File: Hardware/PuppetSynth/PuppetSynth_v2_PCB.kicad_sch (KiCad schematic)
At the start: 59 parts, among them J10 PINHD_1x6_Female, J11 JST_03, J12 JST_03, J13 JST_05, J14 JST_05, J15 JST_05, J16 JST_03, J17 JST_03, J18 JST_03, J19 PINHD_1x6_Female, J20 JST_03, J21 JST_03, J22 JST_03, J24 JST_03, J25 JST_03, J26 JST_03, J3 JST_03, J4 JST_03, J5 JST_05, J6 JST_05, J7 JST_05, J8 PINHD_1x6_Female, J9 PINHD_1x6_Female

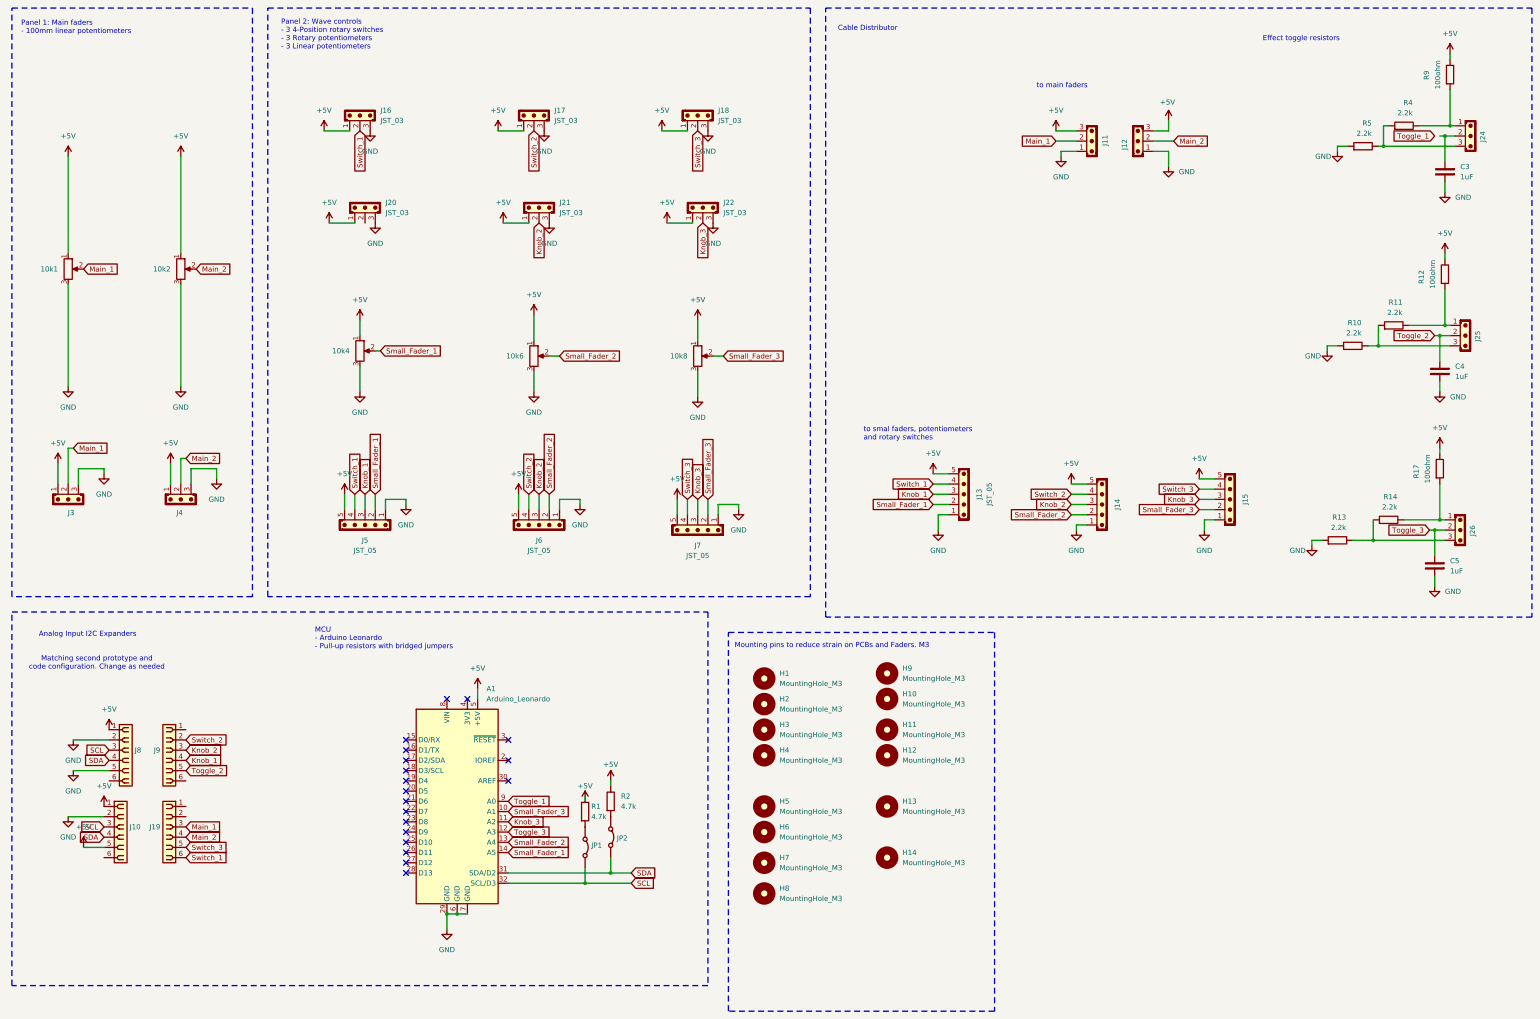
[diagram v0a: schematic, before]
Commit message: updated pcb
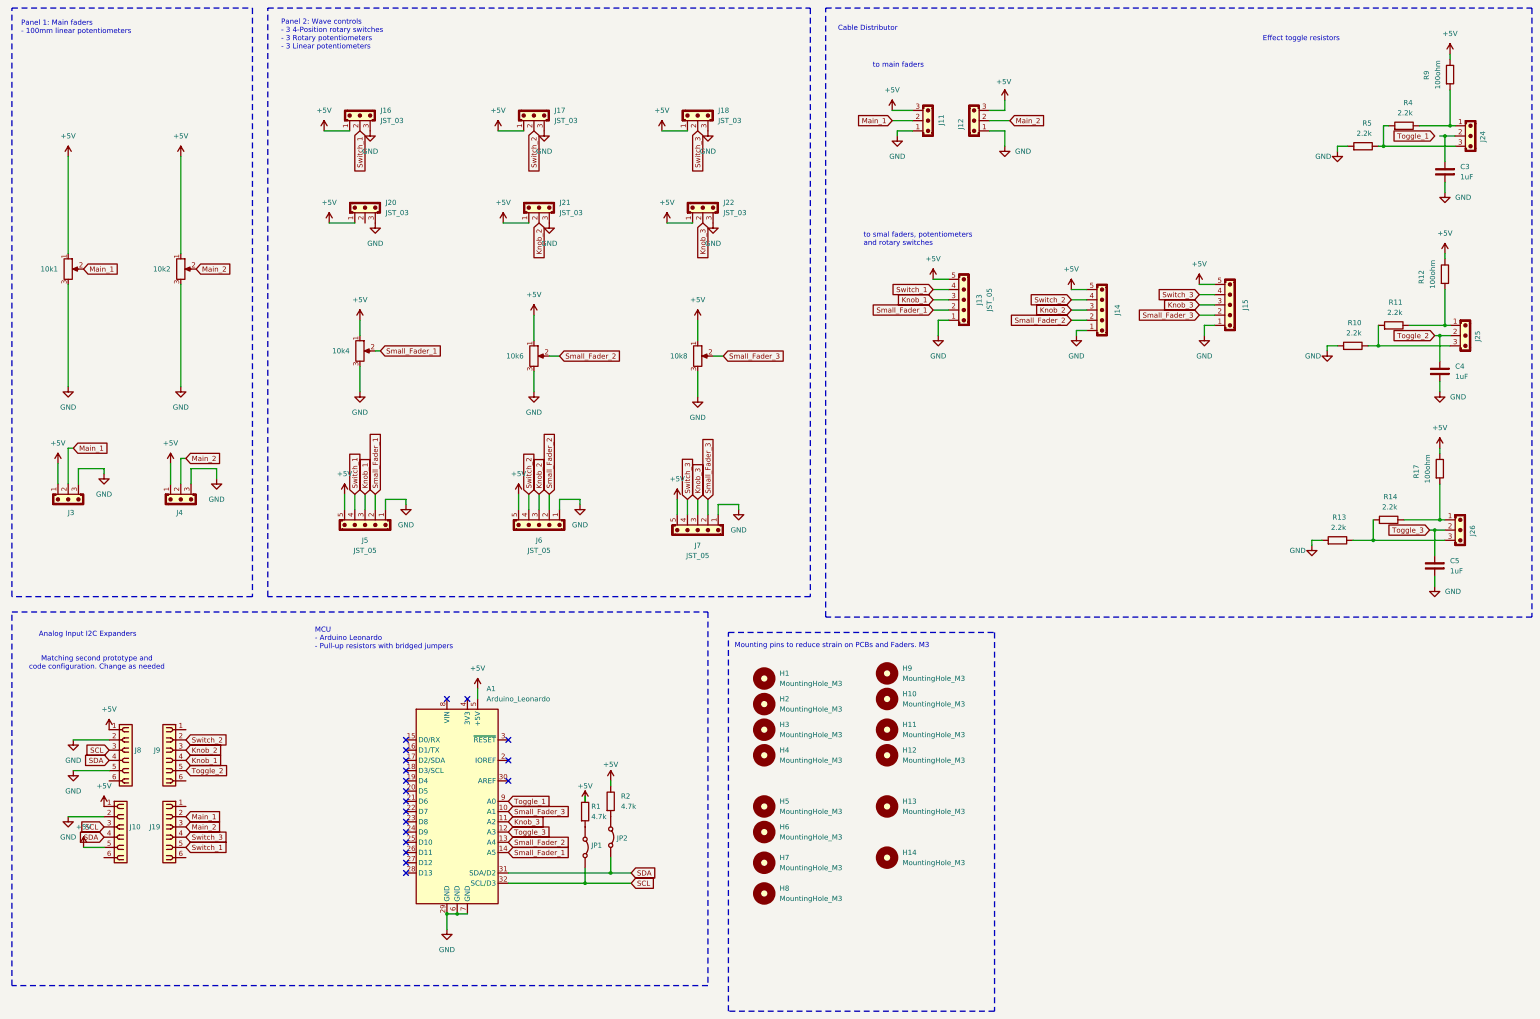
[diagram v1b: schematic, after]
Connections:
- net Main_1: now also J19.2; no longer J19.3
- net Main_2: now also J19.3; no longer J19.4
- net Switch_1: now also J19.5; no longer J19.6
- net Switch_3: now also J19.4; no longer J19.5
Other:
- moved on the sheet: J11, J12, J13, J14, J15
